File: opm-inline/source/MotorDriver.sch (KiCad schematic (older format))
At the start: 38 parts, among them IC1 TMC6200-TA, Q1 HYG025N06LS1C2, Q2 HYG025N06LS1C2, Q3 HYG025N06LS1C2, Q4 HYG025N06LS1C2, Q5 HYG025N06LS1C2, Q6 HYG025N06LS1C2

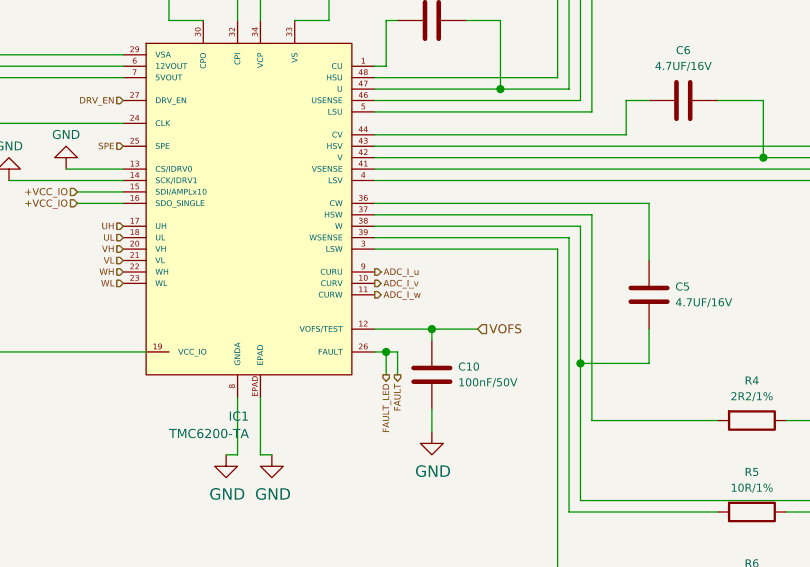
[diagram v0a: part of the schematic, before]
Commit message: rearrange
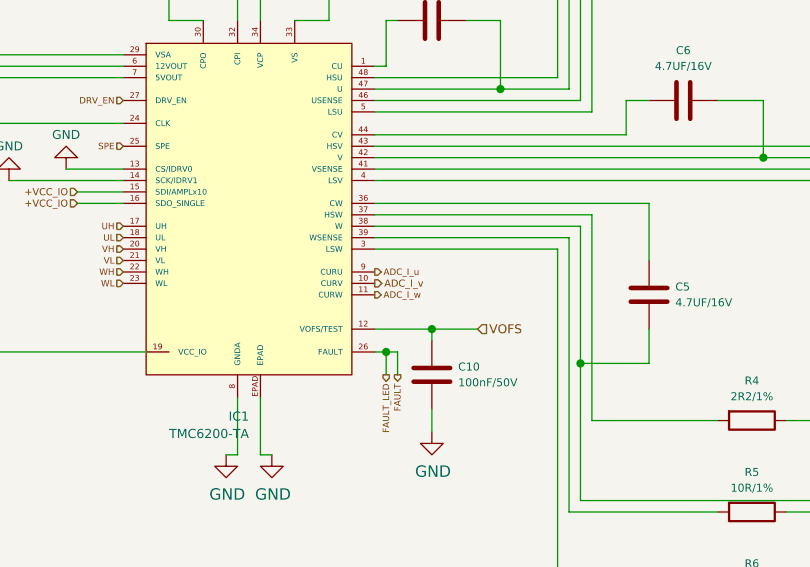
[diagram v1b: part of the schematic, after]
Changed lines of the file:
@@
 Text HLabel 4750 3950 2    28   Output ~ 0
 ADC_I_u
-Text HLabel 4750 4000 2    28   Output ~ 0
-ADC_I_v
 Text HLabel 4750 4050 2    28   Output ~ 0
 ADC_I_w
@@
 	4850 4300 4850 4400
 Connection ~ 4800 4300
+Text HLabel 4750 4000 2    31   Output ~ 0
+ADC_I_v
 $EndSCHEMATC
